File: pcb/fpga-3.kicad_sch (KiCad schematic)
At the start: 5 parts, among them U5 XC7A35T-FGG484

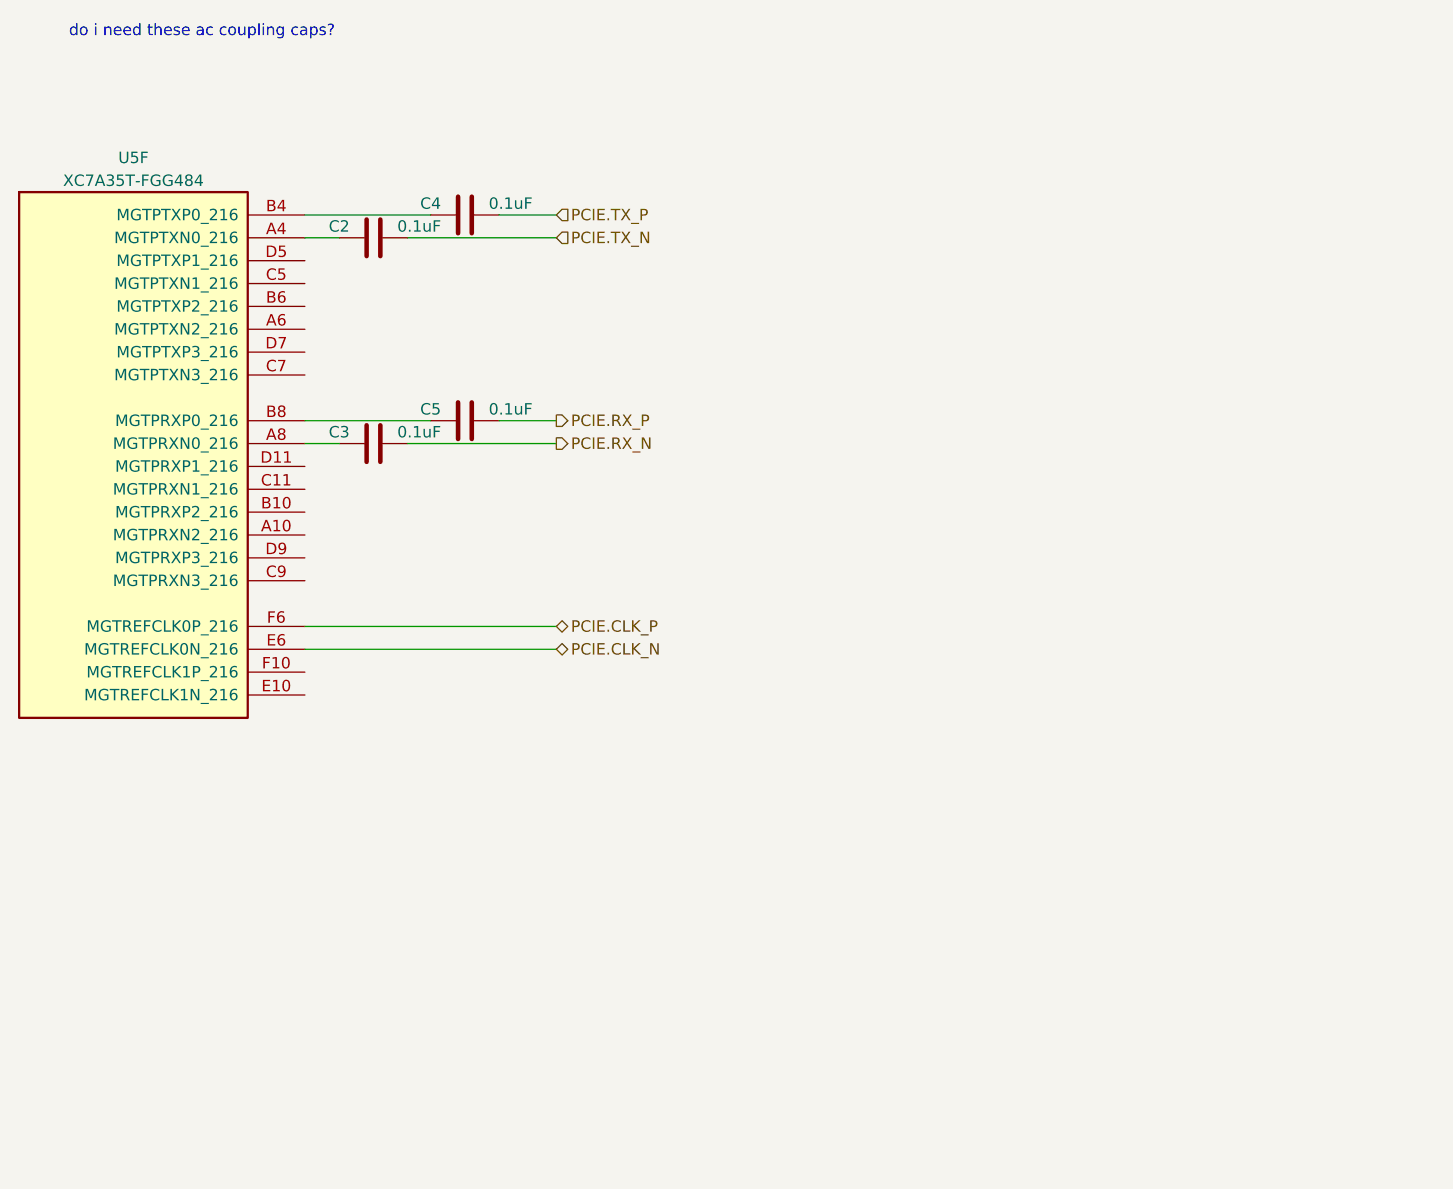
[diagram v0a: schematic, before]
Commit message: pcie definitions
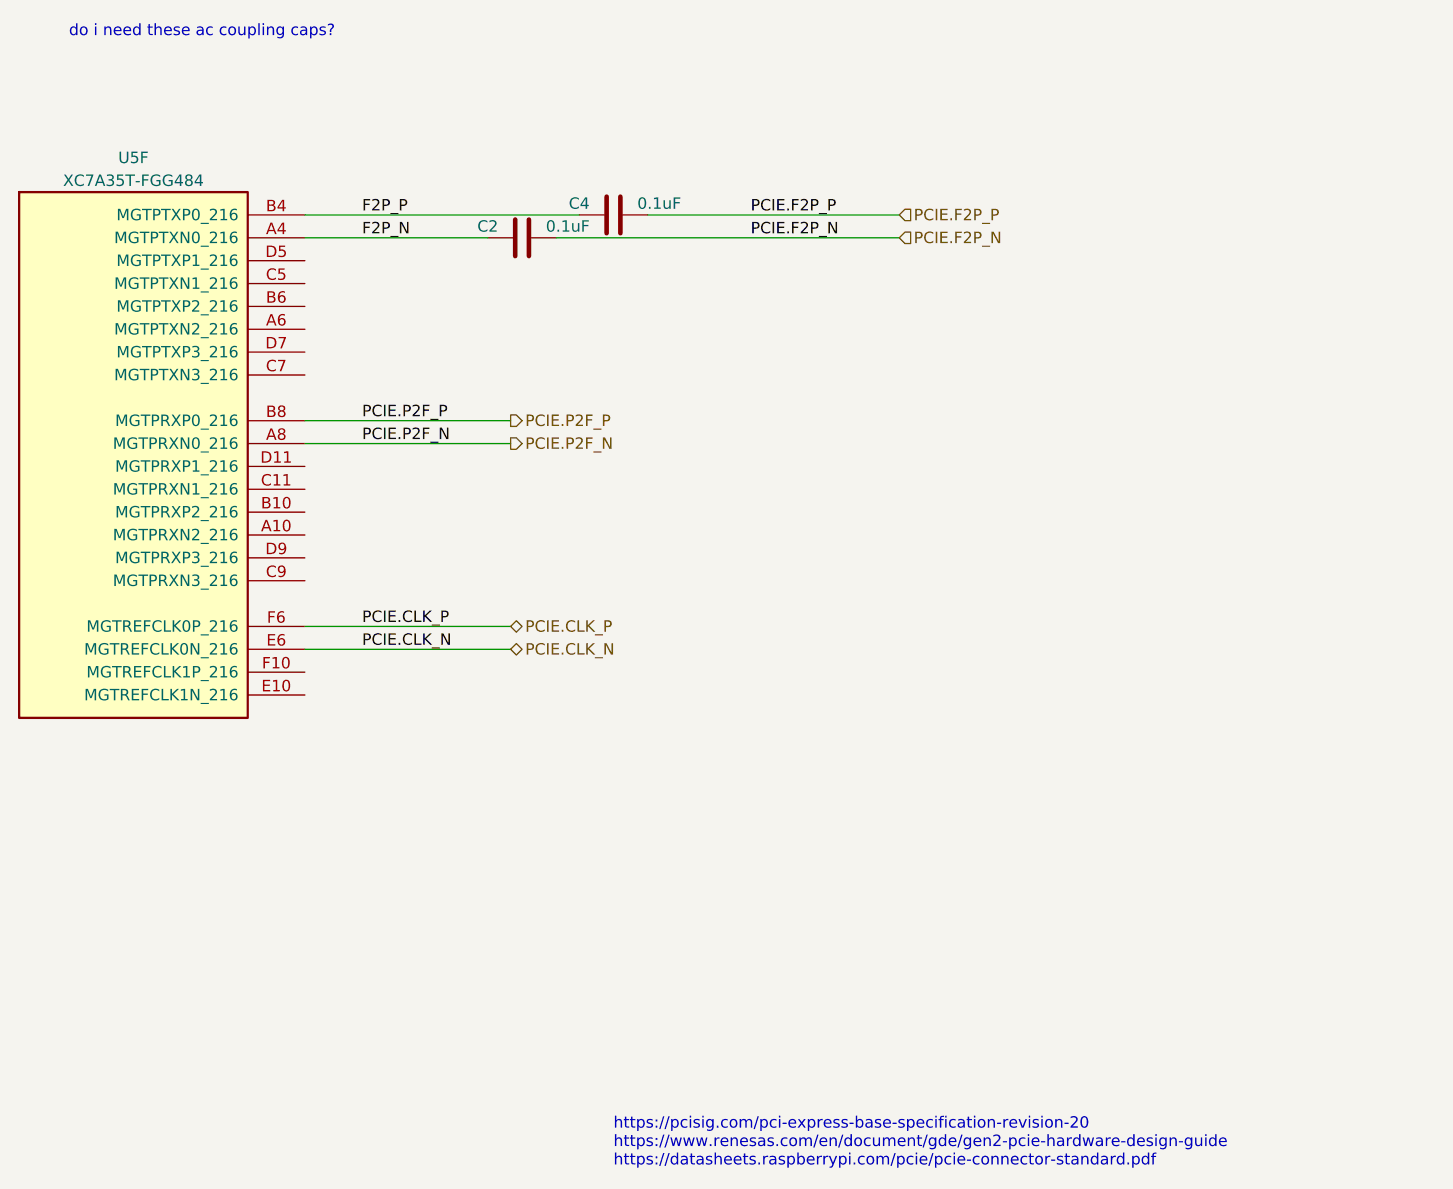
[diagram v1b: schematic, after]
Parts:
- removed C3, C5: 0.1uF, Capacitor_SMD:C_0402_1005Metric, symbol Device:C
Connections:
- net F2P_N: now reaches C2.1, U5.A4 (MGTPTXN0_216)
- net PCIE.P2F_N: now reaches U5.A8 (MGTPRXN0_216)
- net F2P_P: now reaches C4.1, U5.B4 (MGTPTXP0_216)
- net PCIE.P2F_P: now reaches U5.B8 (MGTPRXP0_216)
- net PCIE.TX_N renamed PCIE.F2P_N
- net PCIE.TX_P renamed PCIE.F2P_P
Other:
- note added: "https://pcisig.com/pci-express-base-specification-revision-20 https://www.renesas.com/en/document/gde/gen2-pcie-hardware-design-guide https://datasheets.raspberrypi.com/pcie/pcie-connector-standard.pdf"
- moved on the sheet: C2, C4
